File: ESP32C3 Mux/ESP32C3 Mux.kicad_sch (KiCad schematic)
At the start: 9 parts, among them J1 SSW-104-22-F-D-RA, J2 Conn_01x02_Socket, J3 SSW-104-22-F-D-RA, U1 ESP32C3, U8 STLQ015M33R

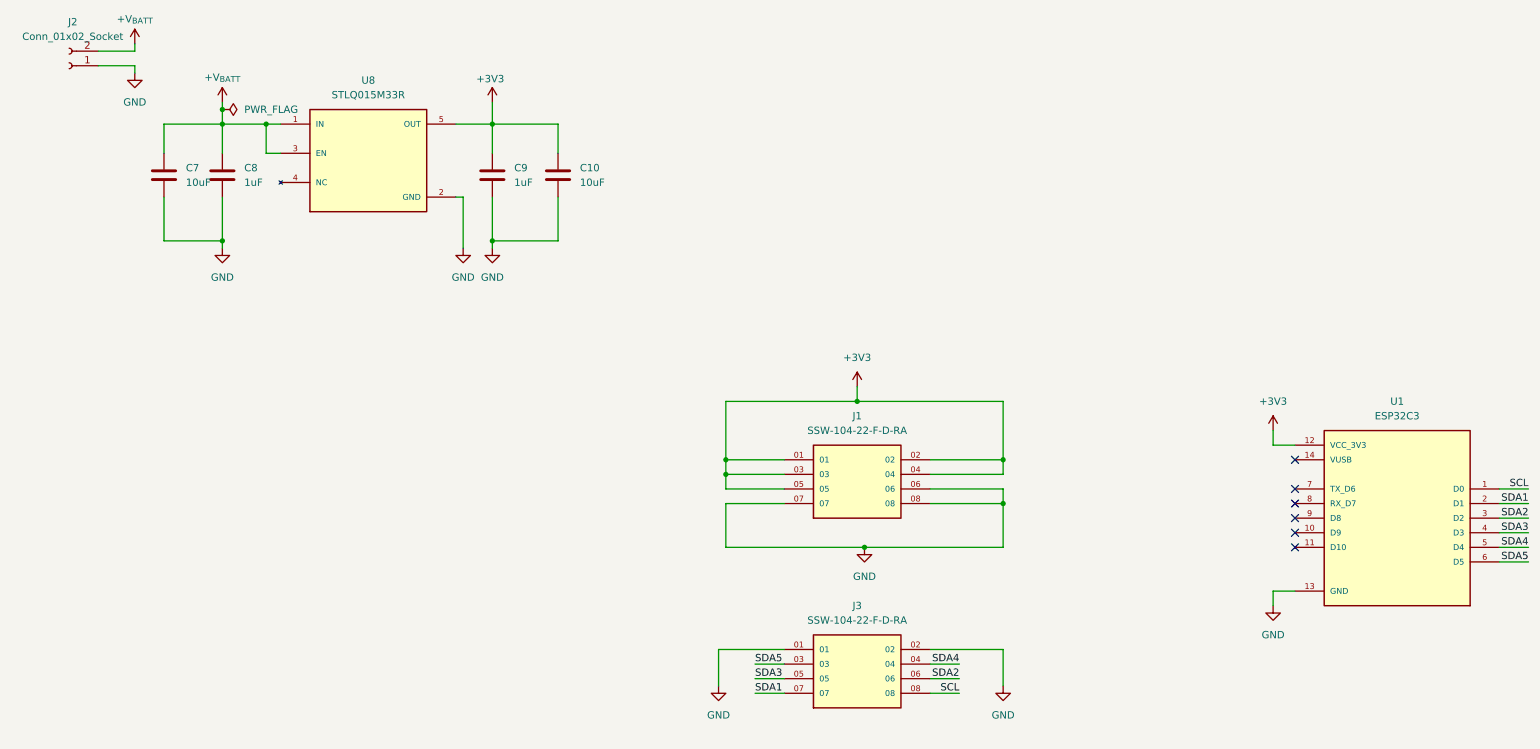
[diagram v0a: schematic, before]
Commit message: updates
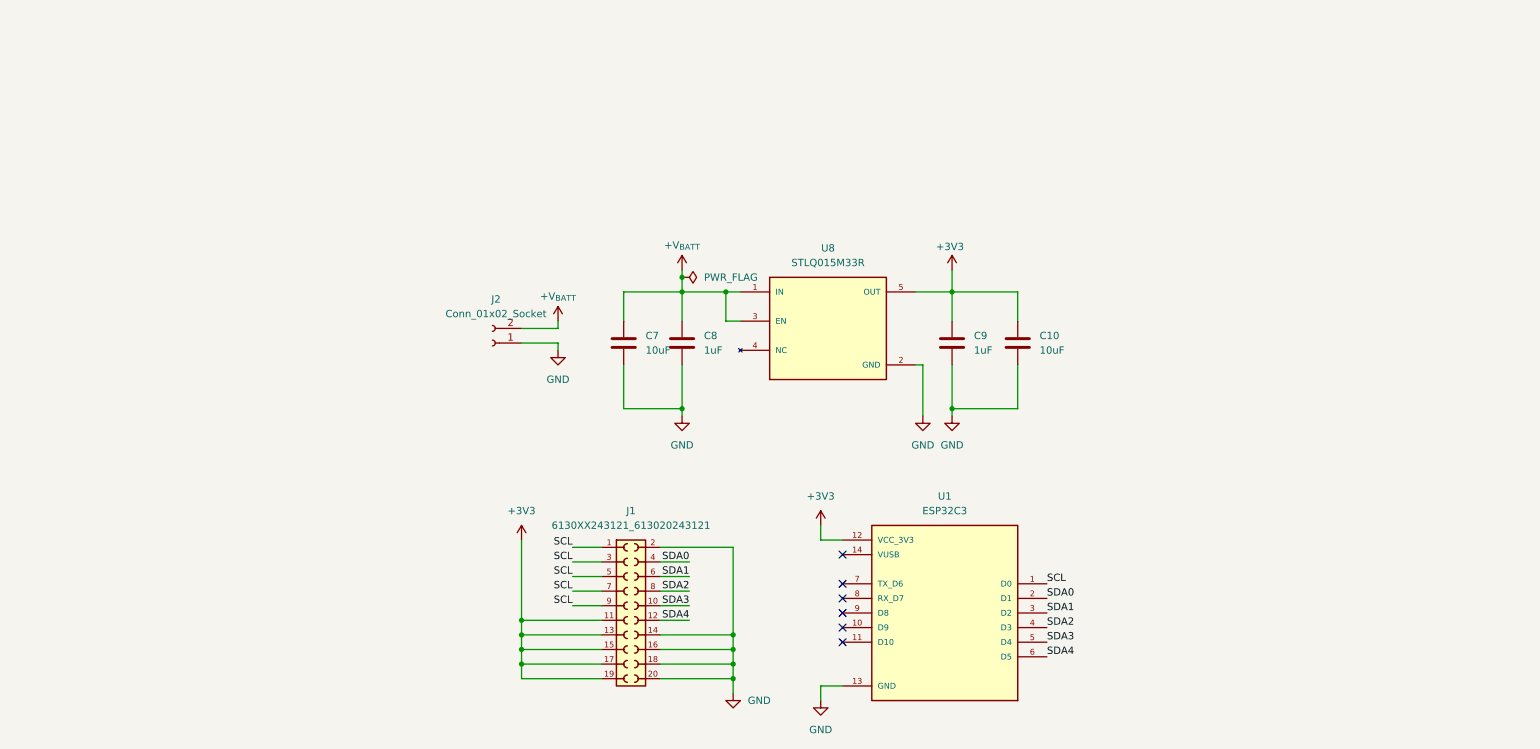
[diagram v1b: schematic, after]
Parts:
- removed J1, J3: SSW-104-22-F-D-RA, ESP32C3 Mux:SAMTEC_SSW-104-22-F-D-RA, symbol ESP32C3Mux:SSW-104-22-F-D-RA
- added J1: 6130XX243121_613020243121, ESP32C3 Mux:613020243121, symbol ESP32C3Mux:6130XX243121_613020243121
- C10, C7, C8, C9: footprint Capacitor_SMD:C_0805_2012Metric -> Capacitor_SMD:C_0805_2012Metric_Pad1.18x1.45mm_HandSolder
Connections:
- net SDA5 is gone; now on net SDA4: U1.6 (D5)
- net +3V3: now also J1.11, J1.13, J1.15, J1.17, J1.19
- net GND: now also J1.14, J1.16, J1.18, J1.2, J1.20
- net SCL: now also J1.1, J1.3, J1.5, J1.7, J1.9
- net SDA1: now also U1.3 (D2), J1.6; no longer U1.2 (D1)
- net SDA2: now also U1.4 (D3), J1.8; no longer U1.3 (D2)
- net SDA3: now also U1.5 (D4), J1.10; no longer U1.4 (D3)
- net SDA4: now also J1.12; no longer U1.5 (D4)
- new net SDA0: J1.4, U1.2 (D1)
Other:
- moved on the sheet: C10, C7, C8, C9, J2, U1, U8
